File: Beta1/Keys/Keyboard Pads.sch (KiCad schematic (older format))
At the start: 27 parts

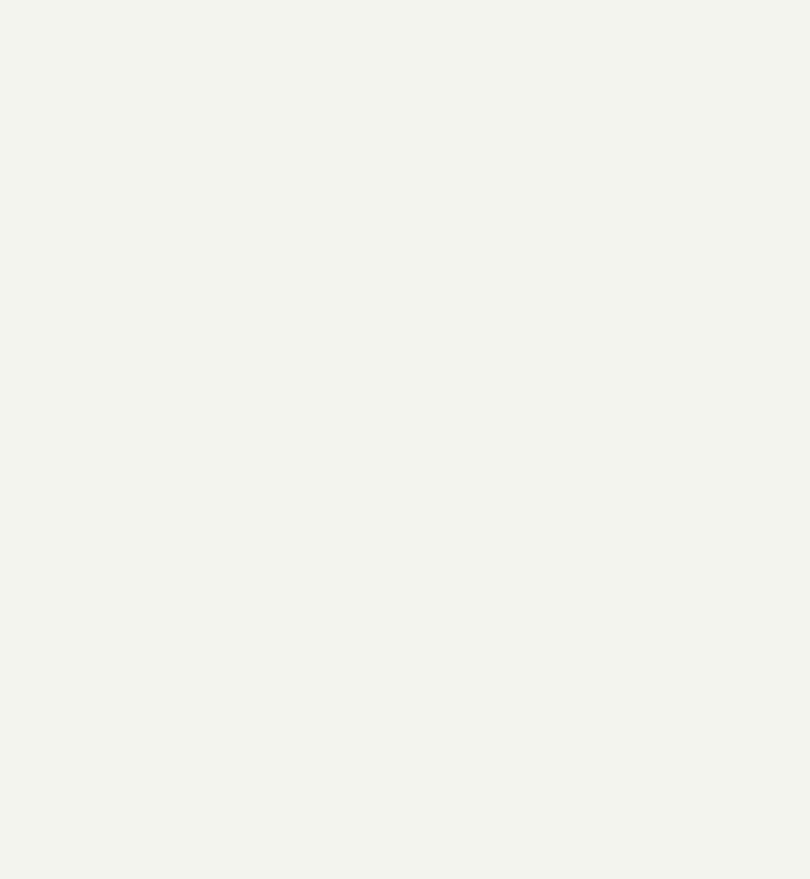
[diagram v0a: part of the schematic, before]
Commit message: Add MPR
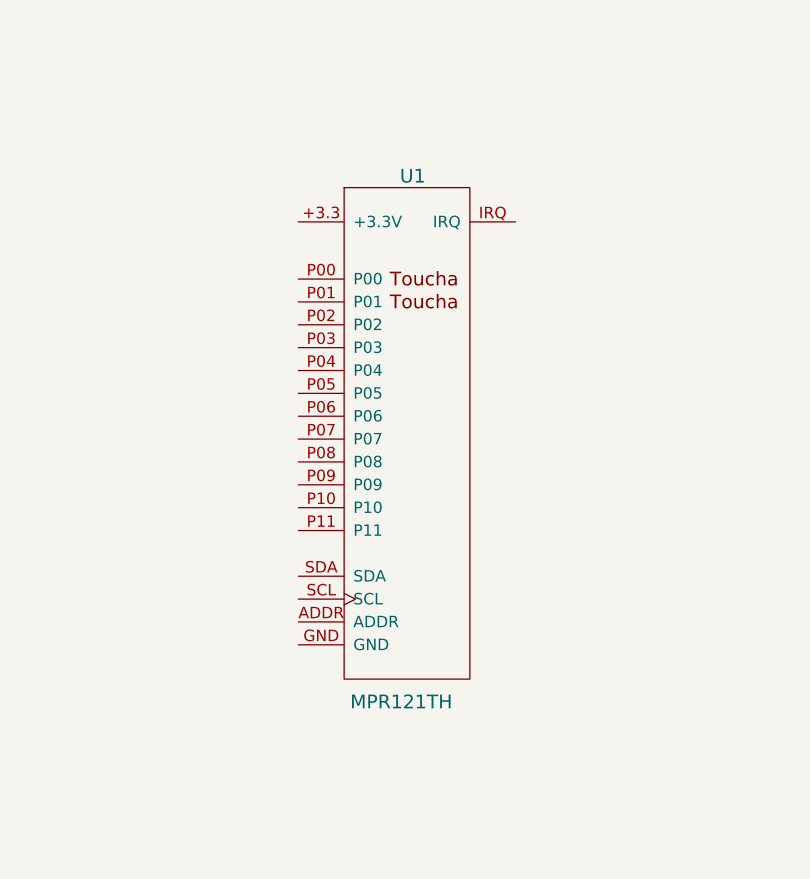
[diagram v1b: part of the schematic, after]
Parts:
- added U1: MPR121TH, Liberry:MPR121TH, symbol MPR121TH
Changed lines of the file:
@@
+	1    0    0    -1
+$EndComp
+$Comp
+L MPR121TH U1
+U 1 1 582FE9DC
+P 10700 3850
+F 0 "U1" H 11000 3900 60  0000 C CNN
+F 1 "MPR121TH" H 10950 1600 60  0000 C CNN
+F 2 "Liberry:MPR121TH" H 10500 2850 60  0001 C CNN
+F 3 "" H 10500 2850 60  0001 C CNN
+F 4 "Believotron" H 10700 3850 60  0001 C CNN "MFG"
+F 5 "BTWLMPR121TH" H 10700 3850 60  0001 C CNN "MPN"
+	1    10700 3850
 	1    0    0    -1
 $EndComp
